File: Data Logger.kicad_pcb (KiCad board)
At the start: 2 copper layers, 50.8 x 30.5 mm, 29 parts, among them J1 CONN_01x04_MALE, J2 CONN_01x09_MALE, J3 CONN_01x04_MALE, J4 CONN_MALE_02X03_ODDEVEN, U1 24LC1025, U2 DS1339U-3+, U3 24LC1025, U4 ATMEGA328P-AU, Y1 32 KHz, Y2 16 MHz

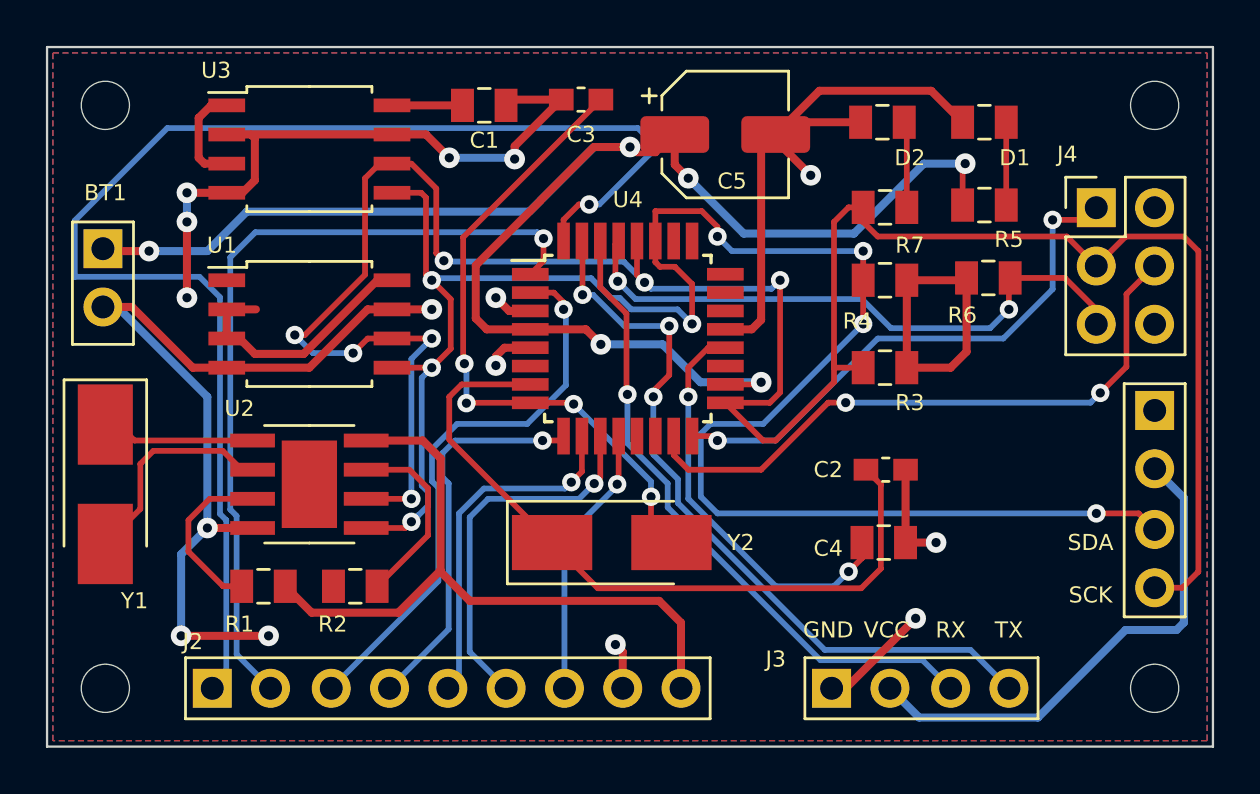
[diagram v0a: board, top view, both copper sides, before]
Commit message: routing
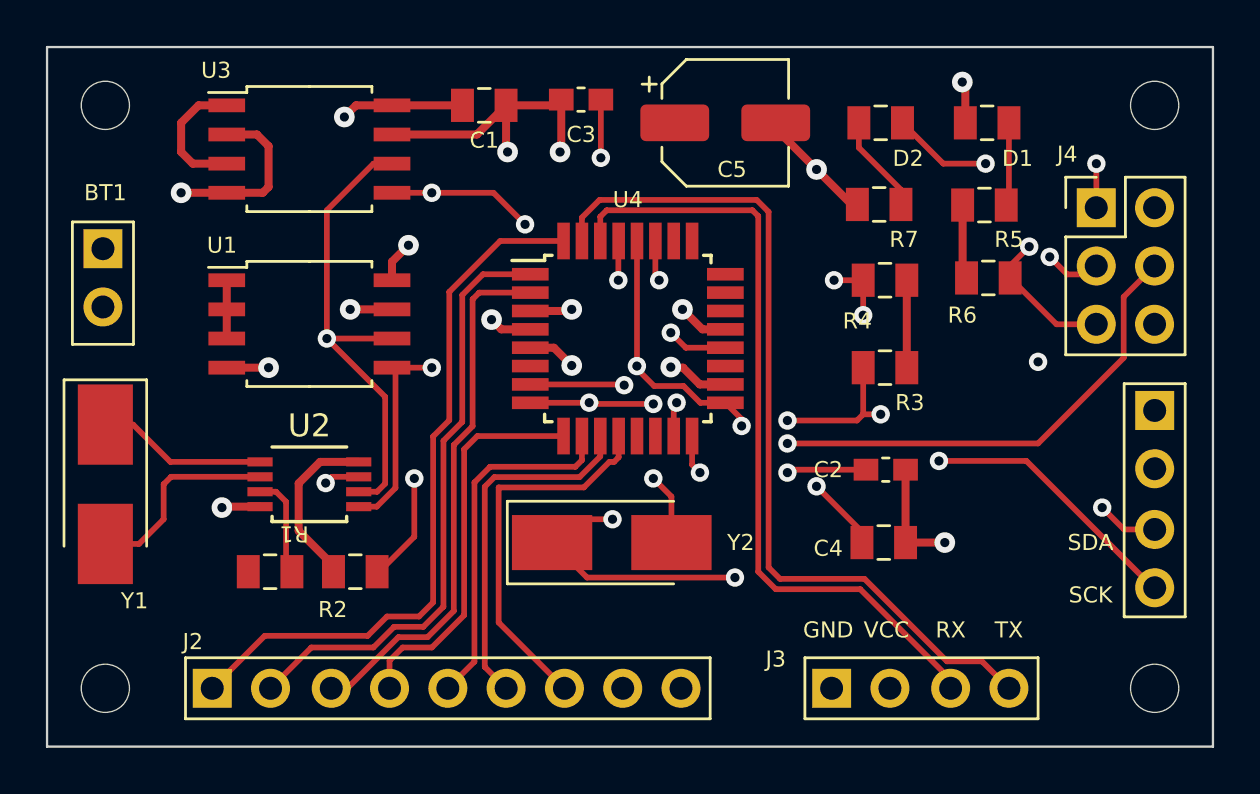
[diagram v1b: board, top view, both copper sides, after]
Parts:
- U2: footprint RN_IC_RTC:U_SMD_DS1339U_DIP08_ANA_DS1339U-3+ -> RN_IC_RTC:U_SMD_DS1339U_TSSOP08_ANA_DS1339U-3+
- moved R1 1.89 mm to (53.2, 83.3), turned to 180 degrees
- moved R7 1.22 mm to (79.2, 68.4), turned to 0 degrees
- moved R2 0.64 mm to (56.9, 83.3)
- moved C5 0.51 mm to (72.7, 64.3)
- moved D1 0.12 mm to (83.9, 64.8)
- moved D2 0.08 mm to (79.2, 64.8)
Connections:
- D2 pad 1: GND -> Net-(D2-Pad1)
- D2 pad 2: Net-(D2-Pad2) -> /SCK
- R7 pad 1: Net-(D2-Pad2) -> GND
- R7 pad 2: /SCK -> Net-(D2-Pad1)
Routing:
- net /Vcc: track 156.6 -> 55.0 mm, vias 6 -> 4
- net GND: track 109.2 -> 43.5 mm, vias 15 -> 12
- net /D2: track 59.9 -> 30.9 mm, vias 1 -> 0
- net /SDA: track 84.4 -> 62.2 mm, vias 8 -> 7
- net /SCK: track 105.9 -> 94.2 mm, vias 7 -> 9
- net /MISO: track 23.7 -> 33.1 mm
- net /D3: track 35.5 -> 26.3 mm, vias 1 -> 0
- net /RX: track 28.4 -> 34.4 mm, vias 1 -> 0
- net /TX: track 32.9 -> 37.8 mm, vias 3 -> 0
- net /D8: track 12.0 -> 16.6 mm, vias 1 -> 0
- net Net-(D2-Pad1): track 0.00 -> 4.32 mm
- net Net-(D2-Pad2): track 3.76 -> 0.00 mm
- net Net-(C3-Pad2): track 28.3 -> 25.2 mm
- net Net-(R1-Pad1): track 7.49 -> 4.47 mm
- net Net-(R2-Pad1): track 8.22 -> 10.3 mm, vias 0 -> 2
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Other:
- copper layers 2 -> 4
